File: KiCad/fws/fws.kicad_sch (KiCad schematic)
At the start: 5 parts, among them J1 Conn_01x03_Socket, J2 Conn_01x03_Socket, U1 RP2040, U2 MIC5205-3.3YM5, U3 W25Q128JVS

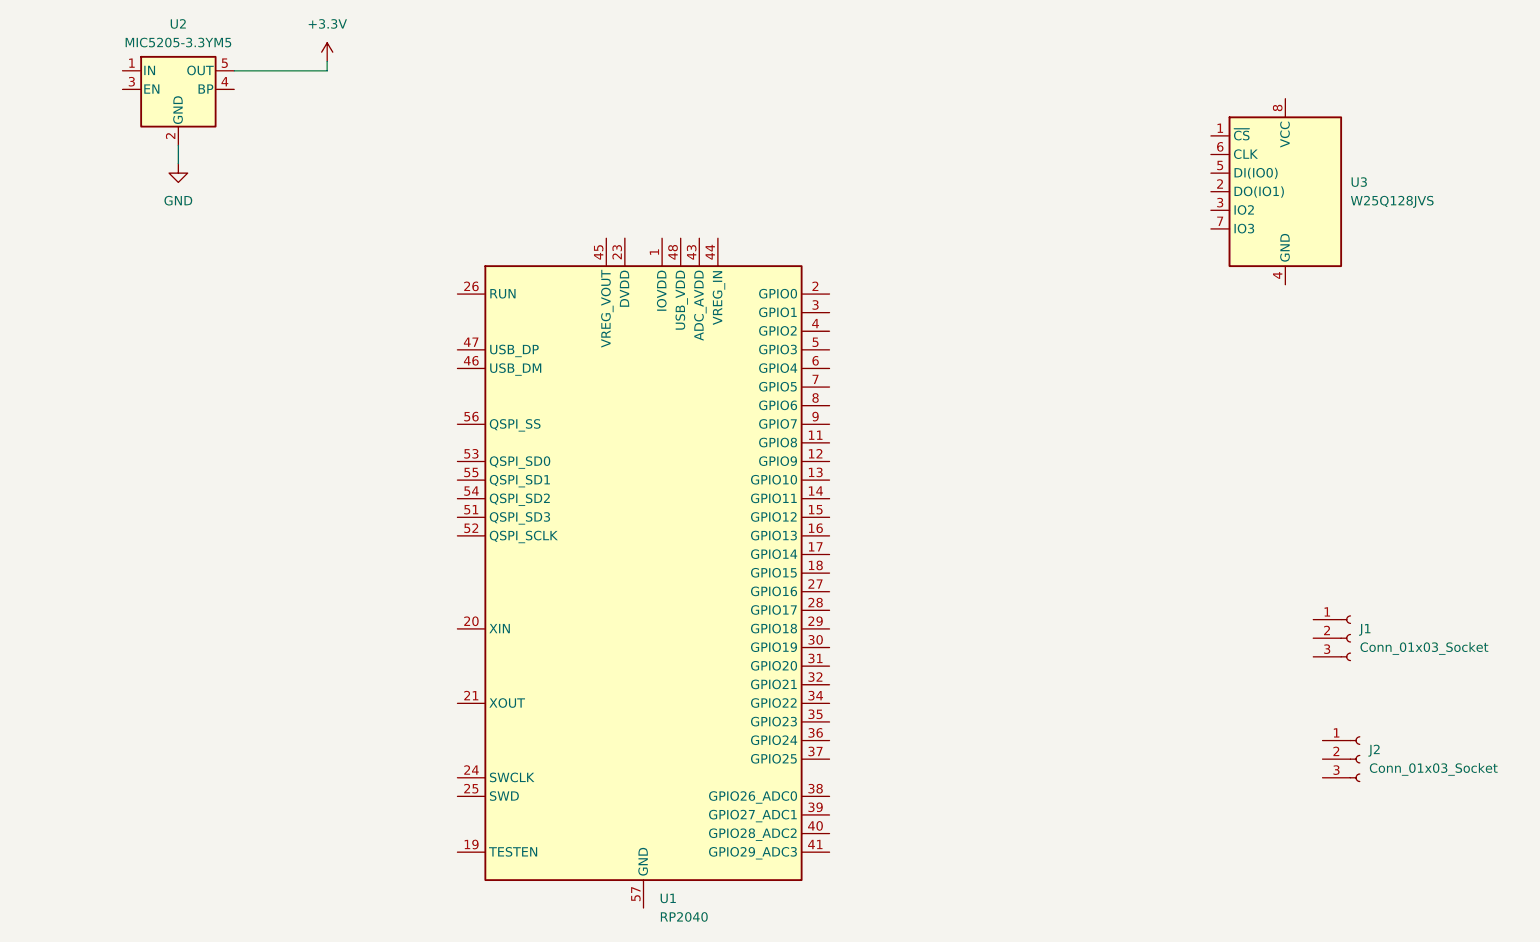
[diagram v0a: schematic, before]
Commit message: Various kicad project updates.
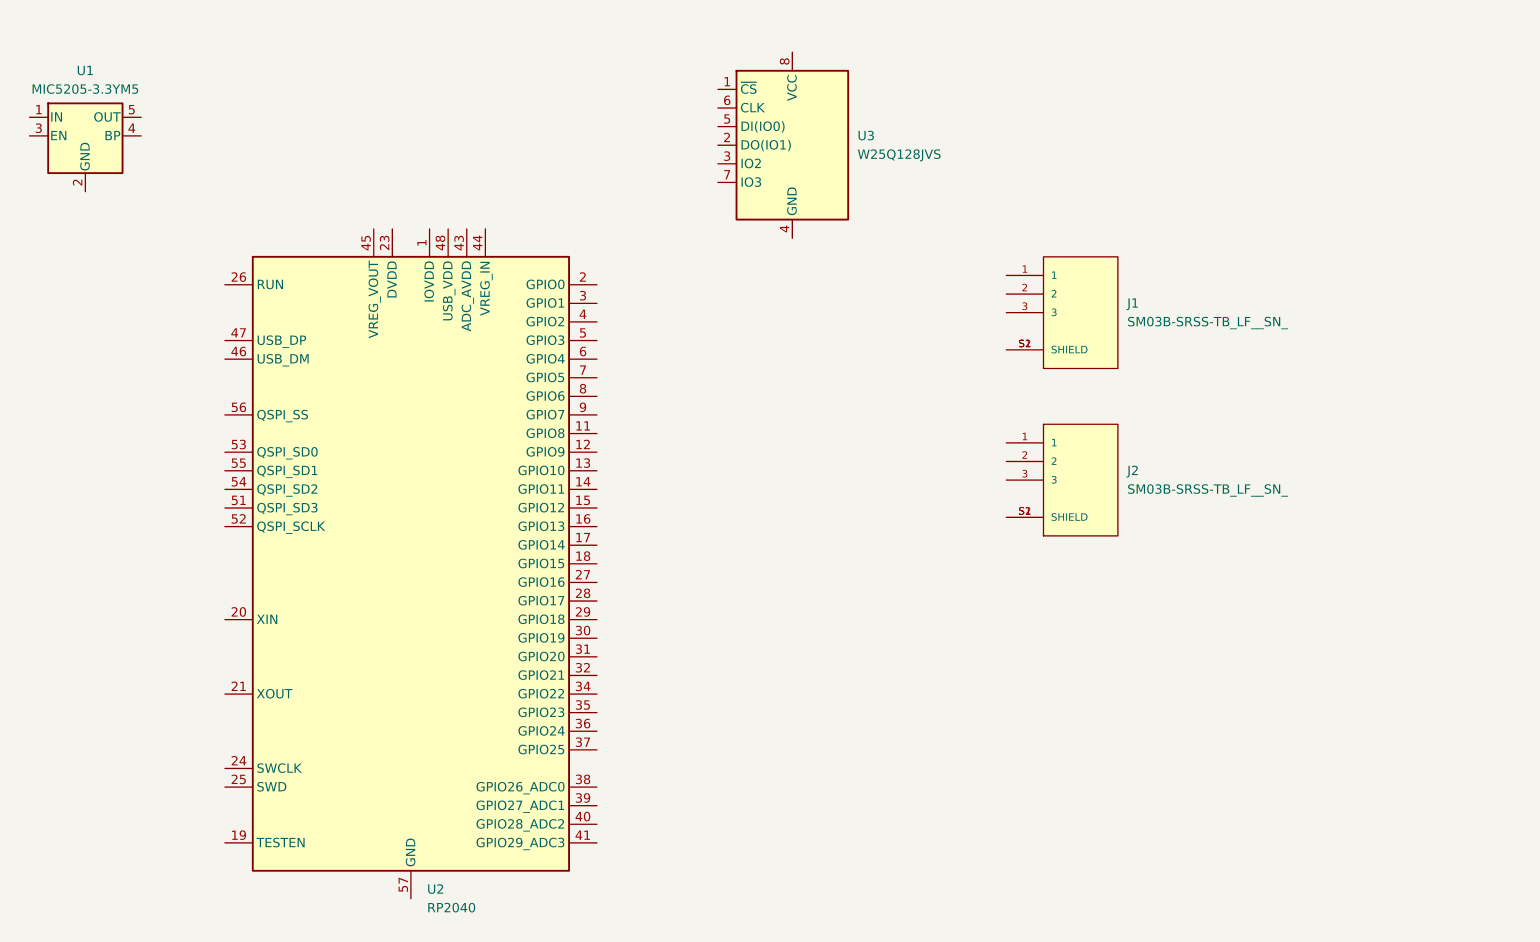
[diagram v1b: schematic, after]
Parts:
- removed J1, J2: Conn_01x03_Socket, symbol Connector:Conn_01x03_Socket
- removed U1: RP2040, Package_DFN_QFN:QFN-56-1EP_7x7mm_P0.4mm_EP3.2x3.2mm, symbol MCU_RaspberryPi:RP2040
- removed U2: MIC5205-3.3YM5, Package_TO_SOT_SMD:SOT-23-5, symbol Regulator_Linear:MIC5205-3.3YM5
- removed U3: W25Q128JVS, Package_SO:SOIC-8_5.23x5.23mm_P1.27mm, symbol Memory_Flash:W25Q128JVS
- added J1, J2: SM03B-SRSS-TB_LF__SN_, fws:SM03B-SRSS-TB_LF__SN_, symbol FWS:SM03B-SRSS-TB_LF__SN_
- added U1: MIC5205-3.3YM5, Package_TO_SOT_SMD:SOT-23-5, symbol FWS:MIC5205-3.3YM5
- added U2: RP2040, Package_DFN_QFN:QFN-56-1EP_7x7mm_P0.4mm_EP3.2x3.2mm, symbol FWS:RP2040
- added U3: W25Q128JVS, Package_SO:SOIC-8_5.23x5.23mm_P1.27mm, symbol FWS:W25Q128JVS
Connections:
- new net: U2.1 (IOVDD), U2.10 (IOVDD), U2.22 (IOVDD), U2.33 (IOVDD), U2.42 (IOVDD), U2.49 (IOVDD)
- new net: U2.23 (DVDD), U2.50 (DVDD)
- new net: J2.S1 (SHIELD), J2.S2 (SHIELD)
- new net: J1.S1 (SHIELD), J1.S2 (SHIELD)
